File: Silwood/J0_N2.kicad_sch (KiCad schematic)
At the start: 19 parts

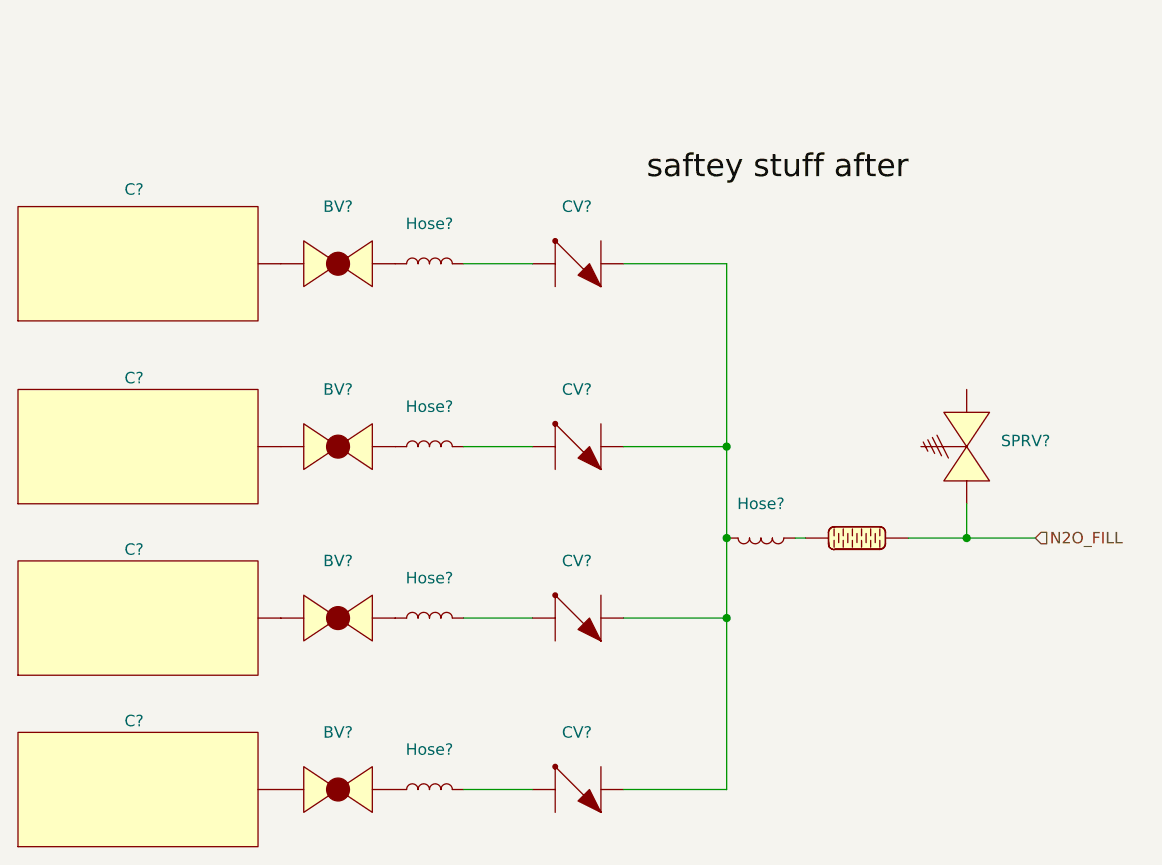
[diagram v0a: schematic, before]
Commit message: update
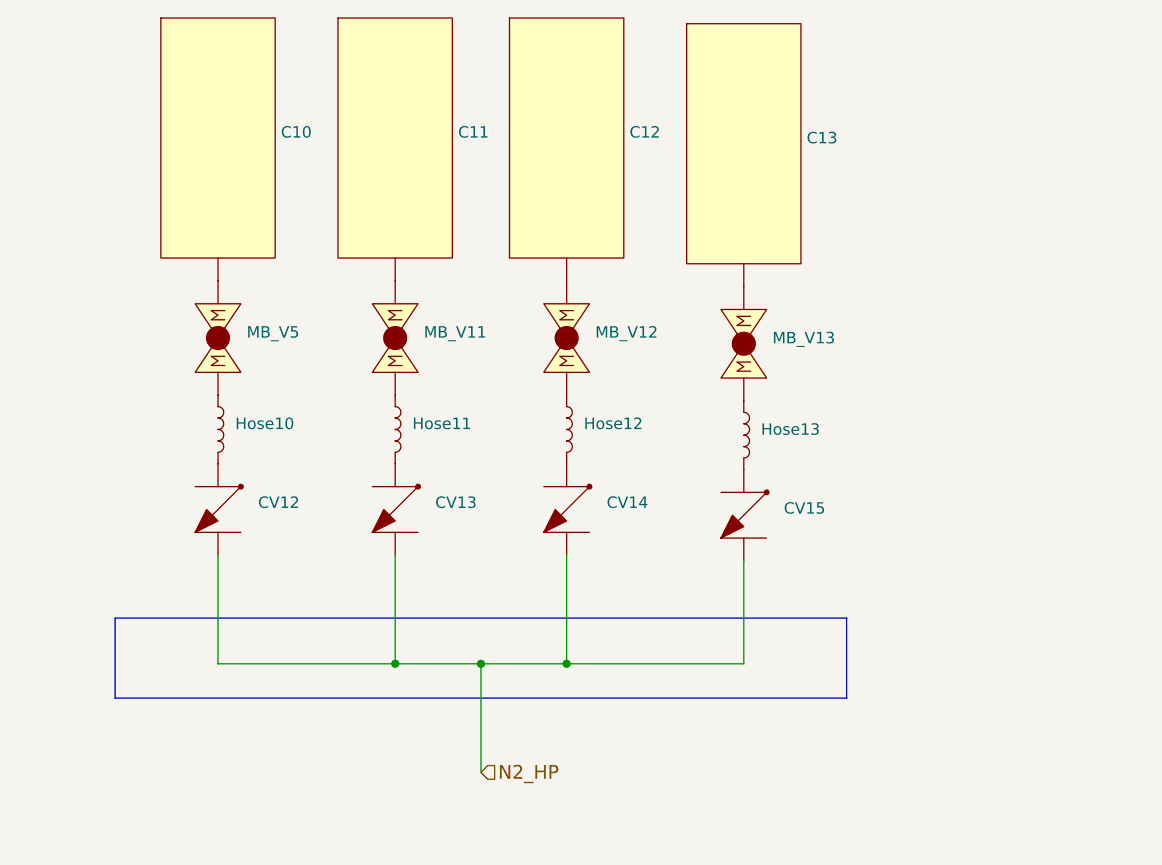
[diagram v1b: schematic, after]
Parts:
- removed BV? (x4): ~, symbol PID_symbols:Ball_Valve
- removed C? (x4): ~, symbol PID_symbols:Cylinder
- removed CV? (x4): ~, symbol PID_symbols:Check_Valve
- removed Filter?: ~, symbol PID_symbols:Filter
- removed Hose? (x5): ~, symbol PID_symbols:Hose
- removed SPRV?: ~, symbol PID_symbols:SPRV
- added C10, C11, C12, C13: ~, symbol PID_symbols:Cylinder
- added CV12, CV13, CV14, CV15: ~, symbol PID_symbols:Check_Valve
- added Hose10, Hose11, Hose12, Hose13: ~, symbol PID_symbols:Hose
- added MB_V11, MB_V12, MB_V13, MB_V5: ~, symbol PID_symbols:MBallValve
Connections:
- new net: CV14., Hose12.
- new net: C10., MB_V5.
- new net: Hose10., MB_V5.
- new net: Hose11., MB_V11.
- new net: CV13., Hose11.
- new net: CV12., Hose10.
- new net: C11., MB_V11.
- new net: C12., MB_V12.
- new net: Hose12., MB_V12.
- new net: CV15., Hose13.
- new net: Hose13., MB_V13.
- new net: C13., MB_V13.
- new net N2_HP: CV12., CV13., CV14., CV15.
